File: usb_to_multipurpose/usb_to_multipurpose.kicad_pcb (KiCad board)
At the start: 2 copper layers, 27 x 30 mm, 39 parts, among them U1 FT232H, U2 AP2112K-3.3TRG1, U5 93LC56BT-I/OT, Y1 12MHz

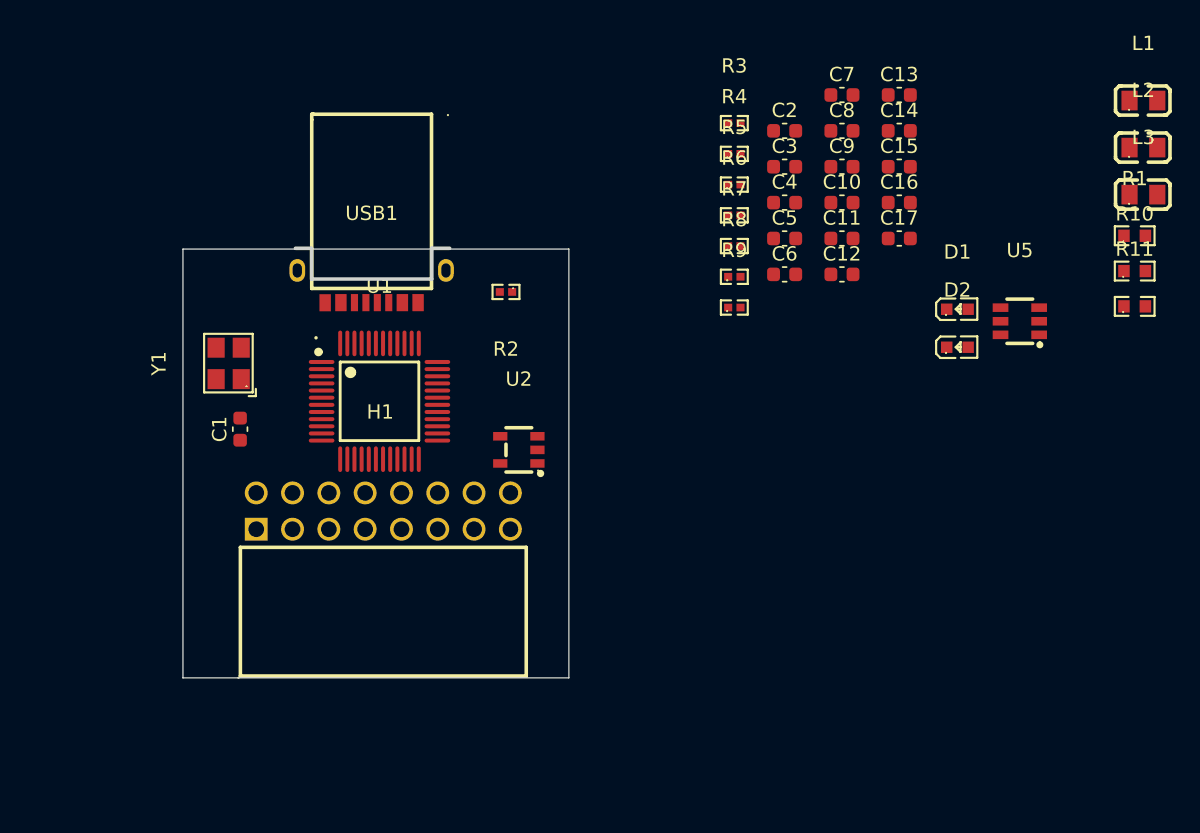
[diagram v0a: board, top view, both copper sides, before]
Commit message: Schematic refinements. Add schematic info.
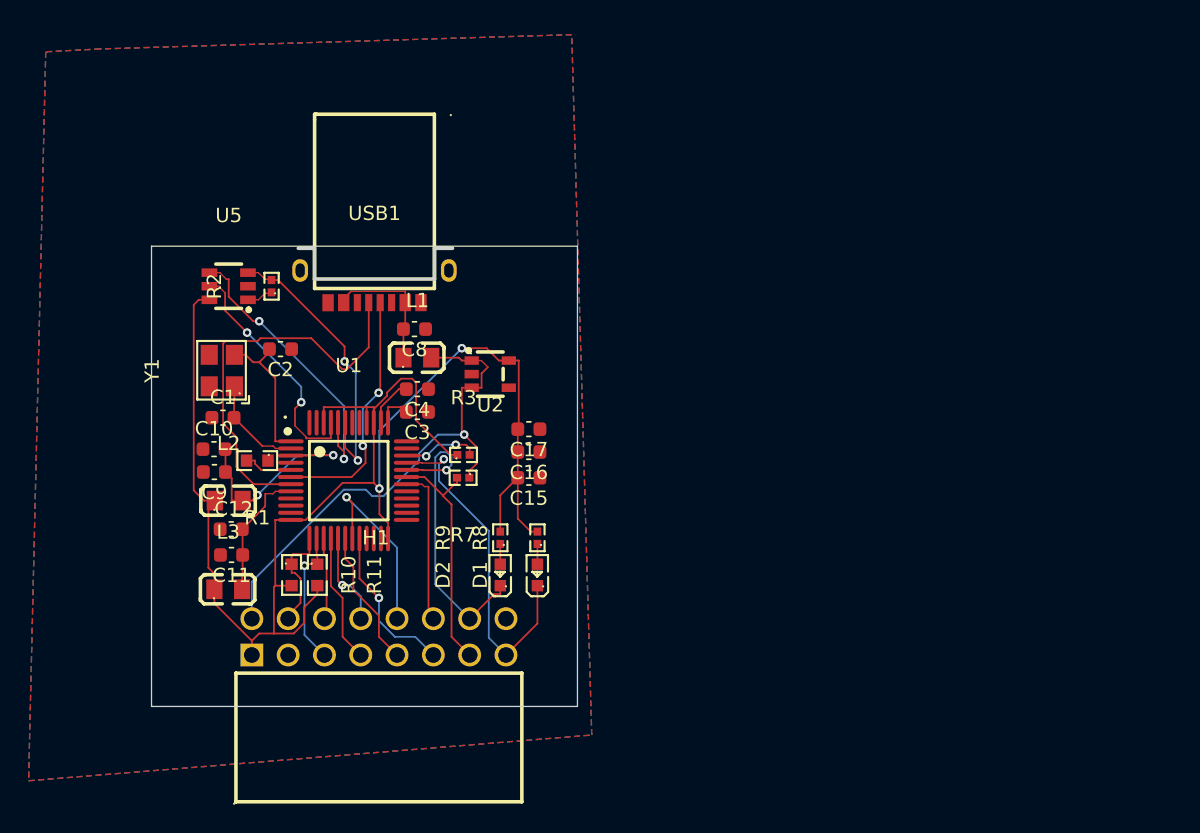
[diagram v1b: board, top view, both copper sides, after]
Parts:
- removed C13, C7: 4.7uF, Capacitor_SMD:C_0603_1608Metric
- removed C14, C5, C6: 0.1uF, Capacitor_SMD:C_0603_1608Metric
- removed R4, R5, R6: 10K, easyeda2kicad:R0402
- moved L3 69.7 mm to (44.4, 58.4)
- moved L2 68.6 mm to (44.4, 52.2)
- moved R1 63.4 mm to (46.4, 49.4), turned to 180 degrees
- moved R10 62.7 mm to (48.8, 57.4), turned to -90 degrees
- moved R11 60.2 mm to (50.6, 57.4), turned to -90 degrees
- moved U5 55.4 mm to (44.4, 37.2)
- moved L1 53.9 mm to (57.6, 42.2)
- moved C9 48.8 mm to (43.4, 50.2), turned to 180 degrees
- moved C11 48.1 mm to (44.6, 56.0), turned to 180 degrees
- moved C10 47.2 mm to (43.4, 48.6)
- moved C12 46.3 mm to (44.6, 54.2)
- moved C2 38.4 mm to (48.0, 41.6), turned to 180 degrees
- moved D2 35.7 mm to (63.4, 57.4), turned to 90 degrees
- moved D1 34.8 mm to (66.0, 57.4), turned to 90 degrees
- moved C15 33.8 mm to (65.4, 50.6), turned to 180 degrees
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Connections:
- H1 pad 12: Net-(U1-ACBUS6) -> Net-(U1-ACBUS5)
- H1 pad 13: Net-(U1-ACBUS7) -> Net-(U1-ACBUS6)
- U1 pad 29: unconnected-(U1-ACBUS5-Pad29) -> Net-(U1-ACBUS5)
- U1 pad 40: VCC -> +5V
- USB1 pad A5: unconnected-(USB1-CC1-PadA5) -> Net-(USB1-CC1)
- USB1 pad B5: unconnected-(USB1-CC2-PadB5) -> Net-(USB1-CC2)
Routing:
- net VCC: track 0.00 -> 111.9 mm, vias 0 -> 2
- net +5V: track 0.00 -> 36.6 mm, vias 0 -> 1
- net /D+: track 0.00 -> 28.3 mm
- net Net-(D1-K): track 0.00 -> 24.3 mm, vias 0 -> 1
- net Net-(D2-K): track 0.00 -> 21.0 mm, vias 0 -> 1
- net Net-(U1-EECLK): track 0.00 -> 20.4 mm, vias 0 -> 2
- net Net-(U1-EEDATA): track 0.00 -> 20.3 mm, vias 0 -> 2
- net /D-: track 0.00 -> 17.4 mm, vias 0 -> 2
- net Net-(U1-EECS): track 0.00 -> 17.0 mm, vias 0 -> 2
- net Net-(U1-ACBUS7): track 0.00 -> 16.8 mm
- net /VPHY: track 0.00 -> 15.3 mm, vias 0 -> 2
- net Net-(U1-ADBUS6): track 0.00 -> 13.0 mm, vias 0 -> 1
- net Net-(U1-ADBUS7): track 0.00 -> 11.1 mm, vias 0 -> 1
- net Net-(U1-ACBUS6): track 0.00 -> 11.0 mm
- net Net-(U1-XCSI): track 0.00 -> 10.3 mm
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- added copper zone on B.Cu, net GND
- added copper zone on F.Cu, net GND
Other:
- board size 27 x 30 mm -> 29.8 x 32.2 mm
